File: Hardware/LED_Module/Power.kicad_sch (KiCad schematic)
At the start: 18 parts, among them U10 AP63203WU, U11 AP63205WU

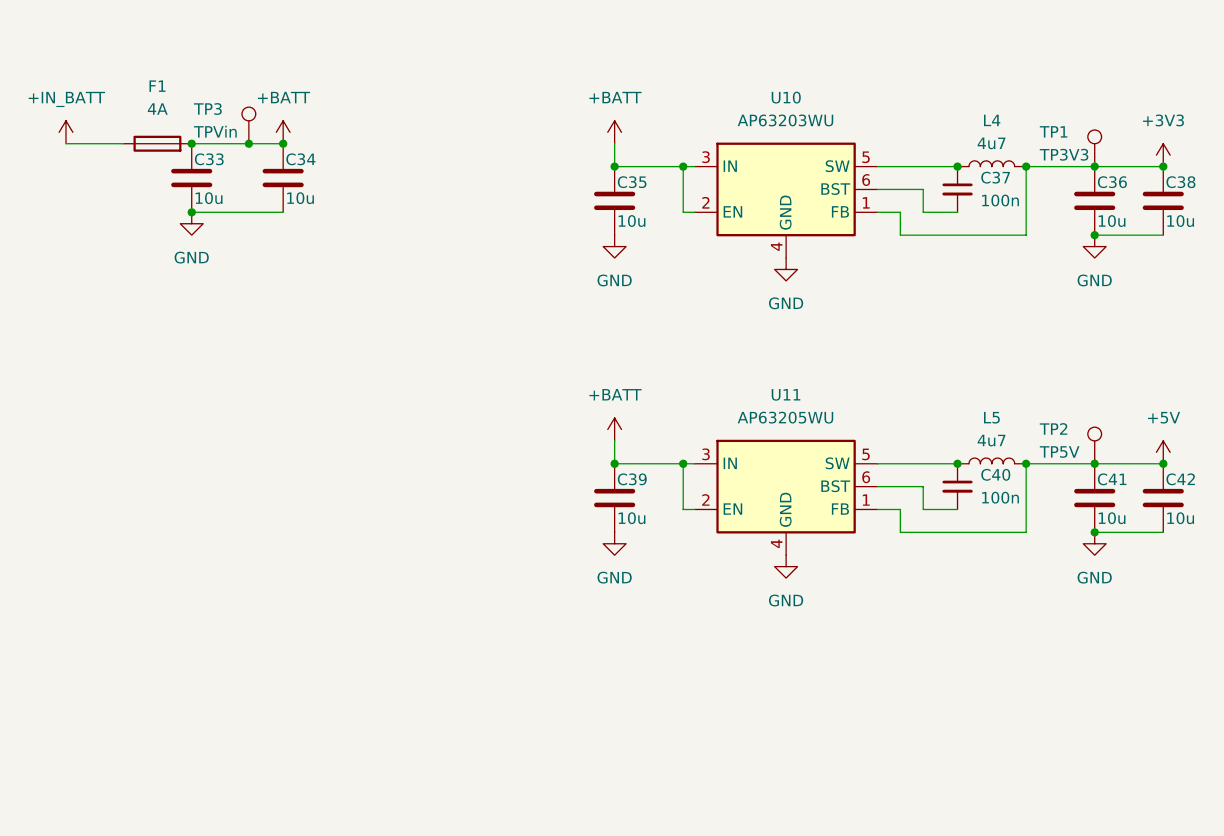
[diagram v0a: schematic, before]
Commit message: La in allt
Myyycket saker
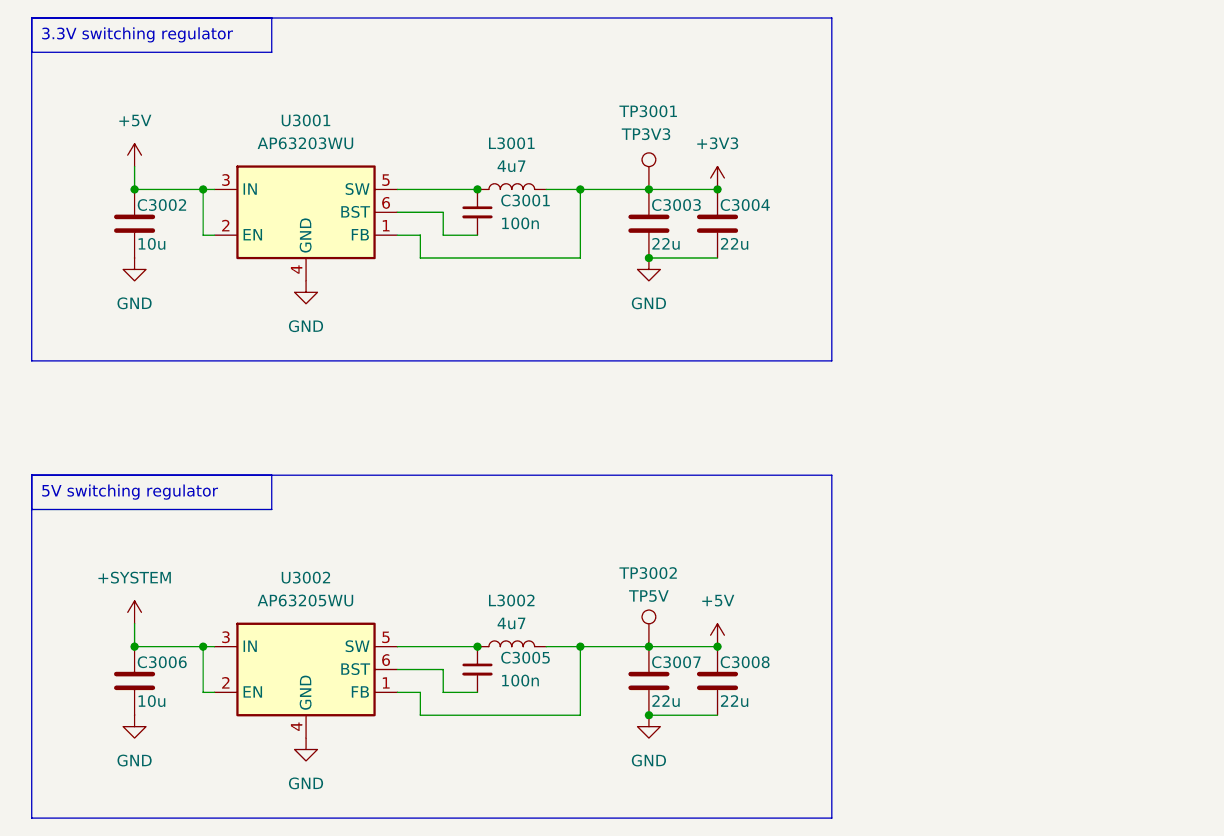
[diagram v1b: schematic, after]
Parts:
- removed C33, C34, C35, C36, C38, C39, C41, C42: 10u, symbol Device:C
- removed C37, C40: 100n, symbol Device:C_Small
- removed F1: 4A, symbol Device:Fuse
- removed L4, L5: 4u7, symbol Device:L
- removed TP1: TP3V3, symbol Connector:TestPoint
- removed TP2: TP5V, symbol Connector:TestPoint
- removed TP3: TPVin, symbol Connector:TestPoint
- removed U10: AP63203WU, Package_TO_SOT_SMD:TSOT-23-6, symbol Regulator_Switching:AP63203WU
- removed U11: AP63205WU, Package_TO_SOT_SMD:TSOT-23-6, symbol Regulator_Switching:AP63205WU
- added C3001, C3005: 100n, Capacitor_SMD:C_0402_1005Metric, symbol Device:C_Small
- added C3002, C3006: 10u, Capacitor_SMD:C_1206_3216Metric, symbol Device:C
- added C3003, C3004, C3007, C3008: 22u, Capacitor_SMD:C_0805_2012Metric, symbol Device:C
- added L3001, L3002: 4u7, Inductor_SMD:L_1210_3225Metric, symbol Device:L
- added TP3001: TP3V3, TestPoint:TestPoint_Pad_D2.0mm, symbol Connector:TestPoint
- added TP3002: TP5V, TestPoint:TestPoint_Pad_D2.0mm, symbol Connector:TestPoint
- added U3001: AP63203WU, Package_TO_SOT_SMD:TSOT-23-6, symbol Regulator_Switching:AP63203WU
- added U3002: AP63205WU, Package_TO_SOT_SMD:TSOT-23-6, symbol Regulator_Switching:AP63205WU
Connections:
- net +3V3: now also C3003.1, C3004.1, L3001.2, TP3001.1, U3001.1 (FB)
- net +5V: now also C3002.1, C3007.1, C3008.1, L3002.2, TP3002.1, U3001.2 (EN), U3001.3 (IN), U3002.1 (FB)
- net GND: now also C3002.2, C3003.2, C3004.2, C3006.2, C3007.2, C3008.2, U3001.4 (GND), U3002.4 (GND)
- new net: C3005.1, L3002.1, U3002.5 (SW)
- new net: C3005.2, U3002.6 (BST)
- new net: C3001.1, L3001.1, U3001.5 (SW)
- new net: C3001.2, U3001.6 (BST)
- new net +SYSTEM: C3006.1, U3002.2 (EN), U3002.3 (IN)
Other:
- company: (none) -> Chalmers EENX16-VT24-27
